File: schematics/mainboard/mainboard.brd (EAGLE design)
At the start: 185 x 110 mm, 145 parts, among them IC1 LM358N, IC2 LM339N, IC3 74AHC00D, IC4 LM2576-5.0, IC5 LM2576-3.3, Q1 BD140, Q2 BD140, Q3 IRF540, T1 2N3904, T2 2N3904, T3 BC847, T4 BC847, T5 BC847, T6 BC847, T7 BC847, T8 BC847, U1 STM32F777VIT, X1 SUPPLY

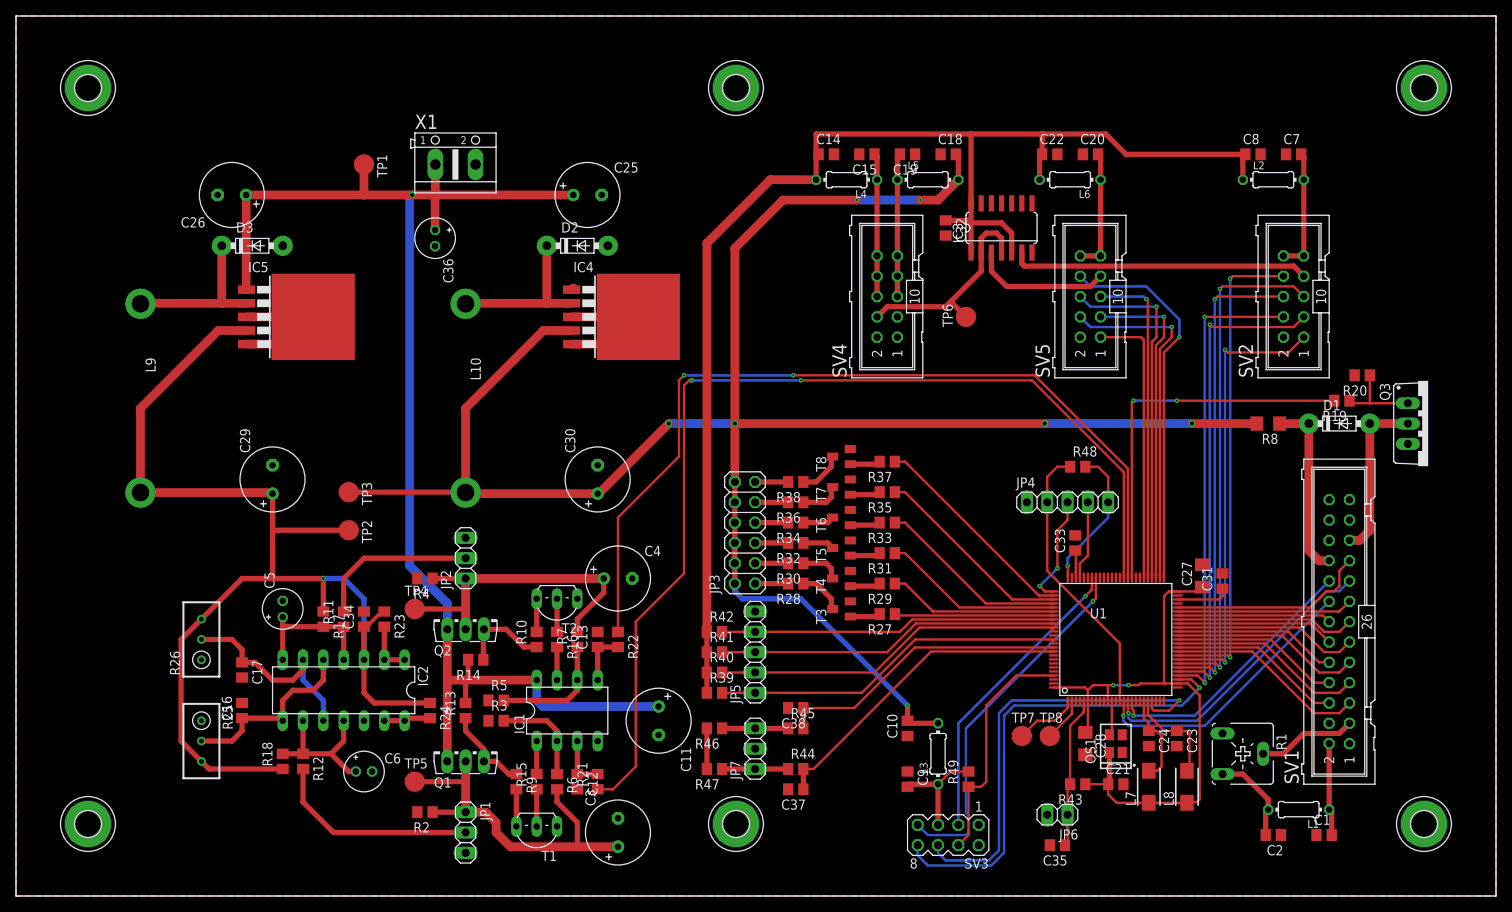
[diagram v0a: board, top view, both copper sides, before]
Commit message: Add files via upload
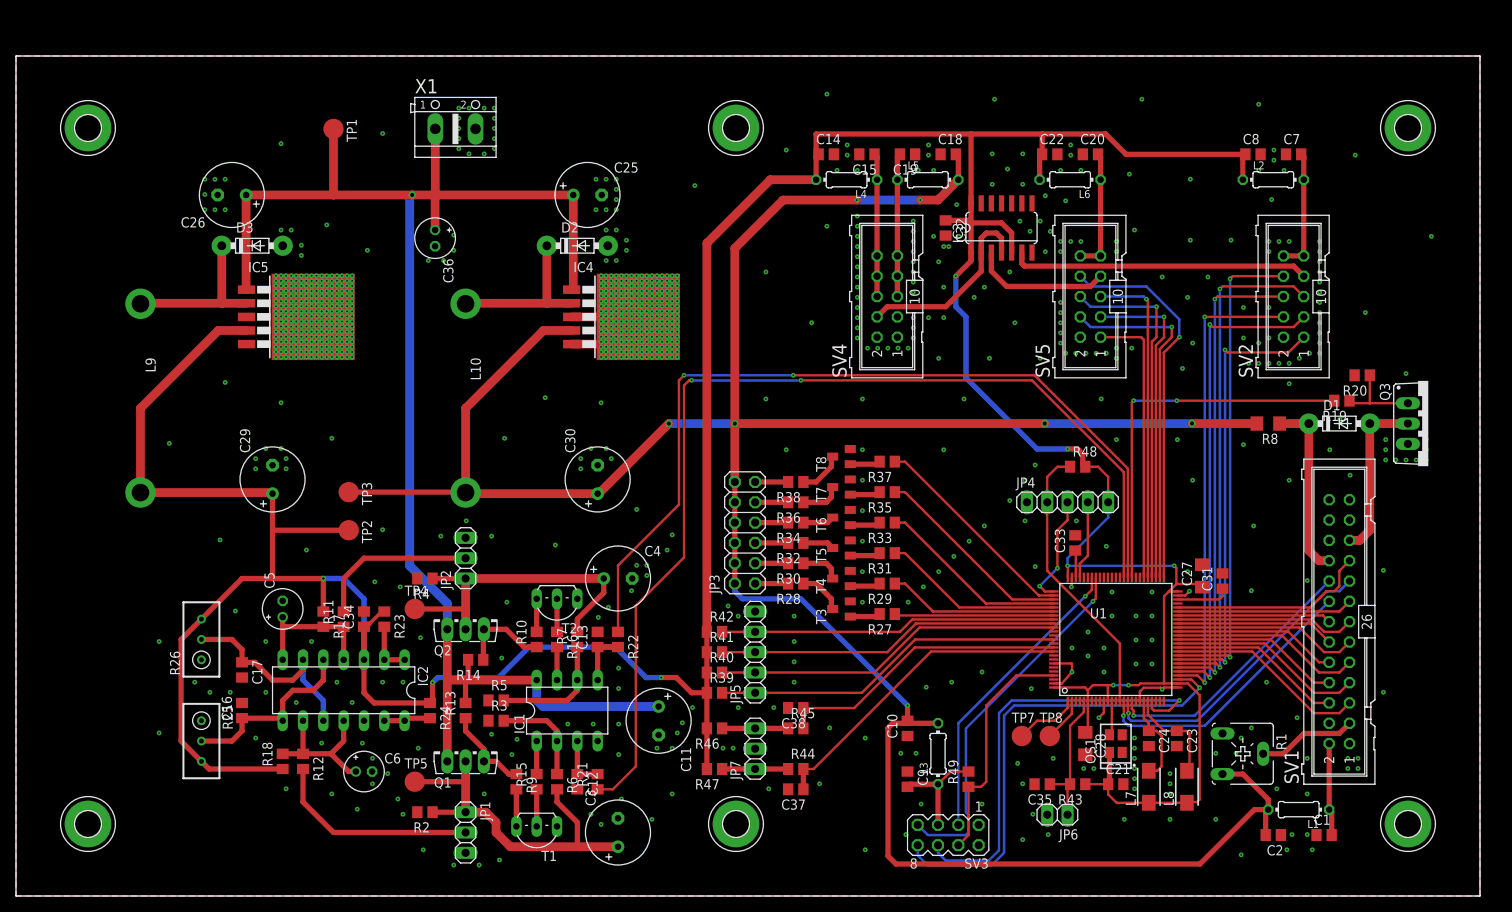
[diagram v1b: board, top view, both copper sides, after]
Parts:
- removed TP6: TPB2,54, testpad:B2,54
- moved C35 7.85 mm to (128.3, 14.0)
- moved TP1 5.85 mm to (39.7, 95.9)
- moved H3 5.39 mm to (174.0, 96.0)
- moved H4 5.00 mm to (9.00, 96.0)
- moved H5 5.00 mm to (90.0, 96.0)
- moved X1 4.45 mm to (54.9, 95.9)
- moved H2 2.00 mm to (174.0, 9.00)
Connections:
- net 32M_REF_OUT: no longer TP6.TP
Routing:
- net +3V3: track 419.8 -> 520.8 mm, vias 4 -> 9
- net +5V: track 267.7 -> 337.4 mm
- net +12V: track 172.7 -> 193.3 mm
- net 32M_REF_OUT: track 27.1 -> 24.4 mm
- net TAMPER: track 18.9 -> 17.5 mm
- net GND: track 35.1 -> 36.0 mm, vias 0 -> 954
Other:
- board size 185 x 110 mm -> 183 x 105 mm
- board text added: "+12V"
- board text added: "+3.3V"
- board text added: "+5V"
- board text added: "ENCODER"
- board text added: "FAN_L"
- board text added: "FAN_R"
- board text added: "FREQ_REFERENCE"
- board text added: "FRONT_SPK/MIC"
- board text added: "KEYBOARD"
- board text added: "LCD_CONNECTOR"
- board text added: "LCD_CONTR"
- board text added: "LEDs"
- board text added: "LEFT"
- board text added: "RIGHT"
- board text added: "RX_BOARD"
- board text added: "SUPPLY"
- board text added: "SWD"
- board text added: "TAMPER"
- board text added: "TP7 8"
- board text added: "TX_BOARD"
- board text added: "V_DN"
- board text added: "V_UP"
